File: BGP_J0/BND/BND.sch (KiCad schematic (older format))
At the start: 7 parts, among them J1 Conn_01x13, J2 Conn_01x03, J3 Conn_01x02, J4 Conn_01x02, J5 Conn_01x03, J6 Conn_01x02, J7 Conn_01x02

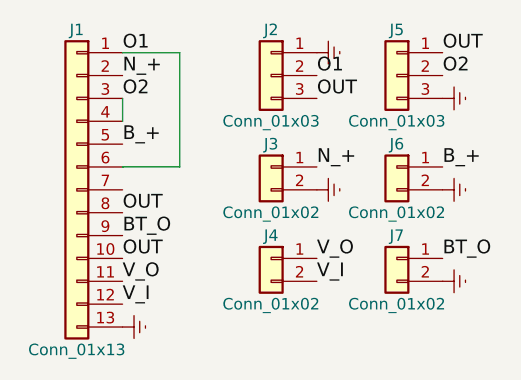
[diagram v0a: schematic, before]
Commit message: Gerbers fixed - ready to go
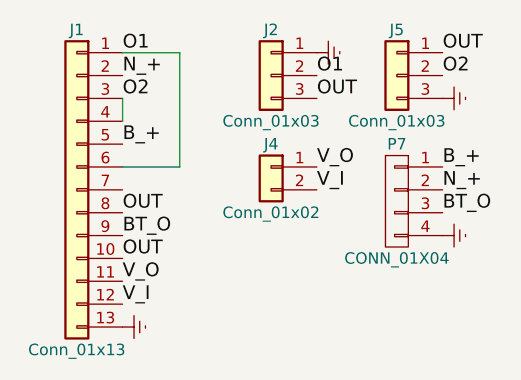
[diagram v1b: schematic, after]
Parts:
- removed J3, J6: Conn_01x02, LIBS:TerminalBlock_Phoenix_MPT-2.54mm_2pol, symbol Conn_01x02
- removed J7: Conn_01x02, Connectors_JST:JST_PH_B2B-PH-K_02x2.00mm_Straight, symbol Conn_01x02
- added P7: CONN_01X04, symbol CONN_01X04
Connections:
- net BT_O: now also P7.3 (P3)
- net B_+: now also P7.1 (P1)
- net Earth: now also P7.4 (P4)
- net N_+: now also P7.2 (P2)
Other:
- moved on the sheet: J4
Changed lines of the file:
@@
 LIBS:switches
 LIBS:relays
-LIBS:motors
 LIBS:transistors
 LIBS:conn
@@
 	-1   0    0    -1
 $EndComp
-$Comp
-L Conn_01x02 J3
-U 1 1 5AE4EB53
-P 5850 3950
-F 0 "J3" H 5850 4050 50  0000 C CNN
-F 1 "Conn_01x02" H 5850 3750 50  0000 C CNN
-F 2 "LIBS:TerminalBlock_Phoenix_MPT-2.54mm_2pol" H 5850 3950 50  0001 C CNN
-F 3 "" H 5850 3950 50  0001 C CNN
-	1    5850 3950
-	-1   0    0    -1
-$EndComp
-$Comp
-L Conn_01x02 J6
-U 1 1 5AE4EB86
-P 6400 3950
-F 0 "J6" H 6400 4050 50  0000 C CNN
-F 1 "Conn_01x02" H 6400 3750 50  0000 C CNN
-F 2 "LIBS:TerminalBlock_Phoenix_MPT-2.54mm_2pol" H 6400 3950 50  0001 C CNN
-F 3 "" H 6400 3950 50  0001 C CNN
-	1    6400 3950
-	-1   0    0    -1
-$EndComp
-Text Label 6050 3950 0    60   ~ 0
+Text Label 6600 4050 0    60   ~ 0
 N_+
 Text Label 5200 3550 0    60   ~ 0
 N_+
-$Comp
-L Earth #PWR01
-U 1 1 5AE4EC05
-P 6050 4050
-F 0 "#PWR01" H 6050 3800 50  0001 C CNN
-F 1 "Earth" H 6050 3900 50  0001 C CNN
-F 2 "" H 6050 4050 50  0001 C CNN
-F 3 "" H 6050 4050 50  0001 C CNN
-	1    6050 4050
-	0    -1   1    0
-$EndComp
-$Comp
-L Earth #PWR02
-U 1 1 5AE4EC20
-P 6600 4050
-F 0 "#PWR02" H 6600 3800 50  0001 C CNN
-F 1 "Earth" H 6600 3900 50  0001 C CNN
-F 2 "" H 6600 4050 50  0001 C CNN
-F 3 "" H 6600 4050 50  0001 C CNN
-	1    6600 4050
-	0    -1   1    0
-$EndComp
 Wire Wire Line
 	5200 3650 5200 3750
@@
 L Conn_01x02 J4
 U 1 1 5AE4EEB8
-P 5850 4350
-F 0 "J4" H 5850 4450 50  0000 C CNN
-F 1 "Conn_01x02" H 5850 4150 50  0000 C CNN
-F 2 "Connectors_JST:JST_PH_B2B-PH-K_02x2.00mm_Straight" H 5850 4350 50  0001 C CNN
-F 3 "" H 5850 4350 50  0001 C CNN
-	1    5850 4350
+P 5850 3950
+F 0 "J4" H 5850 4050 50  0000 C CNN
+F 1 "Conn_01x02" H 5850 3750 50  0000 C CNN
+F 2 "Connectors_JST:JST_PH_B2B-PH-K_02x2.00mm_Straight" H 5850 3950 50  0001 C CNN
+F 3 "" H 5850 3950 50  0001 C CNN
+	1    5850 3950
 	-1   0    0    -1
 $EndComp
-Text Label 6050 4450 0    60   ~ 0
+Text Label 6050 4050 0    60   ~ 0
 V_I
-Text Label 6050 4350 0    60   ~ 0
+Text Label 6050 3950 0    60   ~ 0
 V_O
-$Comp
-L Conn_01x02 J7
-U 1 1 5AE4F048
-P 6400 4350
-F 0 "J7" H 6400 4450 50  0000 C CNN
-F 1 "Conn_01x02" H 6400 4150 50  0000 C CNN
-F 2 "Connectors_JST:JST_PH_B2B-PH-K_02x2.00mm_Straight" H 6400 4350 50  0001 C CNN
-F 3 "" H 6400 4350 50  0001 C CNN
-	1    6400 4350
-	-1   0    0    -1
-$EndComp
-Text Label 6600 4350 0    60   ~ 0
+Text Label 6600 4150 0    60   ~ 0
 BT_O
 $Comp
 L Earth #PWR04
 U 1 1 5AE4F0BF
-P 6600 4450
-F 0 "#PWR04" H 6600 4200 50  0001 C CNN
-F 1 "Earth" H 6600 4300 50  0001 C CNN
-F 2 "" H 6600 4450 50  0001 C CNN
-F 3 "" H 6600 4450 50  0001 C CNN
-	1    6600 4450
+P 6600 4250
+F 0 "#PWR04" H 6600 4000 50  0001 C CNN
+F 1 "Earth" H 6600 4100 50  0001 C CNN
+F 2 "" H 6600 4250 50  0001 C CNN
+F 3 "" H 6600 4250 50  0001 C CNN
+	1    6600 4250
 	0    -1   -1   0
 $EndComp
@@
 Text Label 6600 3550 0    60   ~ 0
 O2
+$Comp
+L CONN_01X04 P7
+U 1 1 5AE6AC54
+P 6400 4100
+F 0 "P7" H 6400 4350 50  0000 C CNN
+F 1 "CONN_01X04" H 6400 3850 50  0000 C CNN
+F 2 "" H 6400 4100 50  0000 C CNN
+F 3 "" H 6400 4100 50  0000 C CNN
+	1    6400 4100
+	-1   0    0    -1
+$EndComp
 $EndSCHEMATC
